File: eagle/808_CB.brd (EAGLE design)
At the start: 100 x 80 mm, 56 parts, among them IC1 4584N, IC2 TL072P, Q1 2N3904, Q2 2N3904, Q3 2N3904, Q4 2N3906, X1 22-23-2021

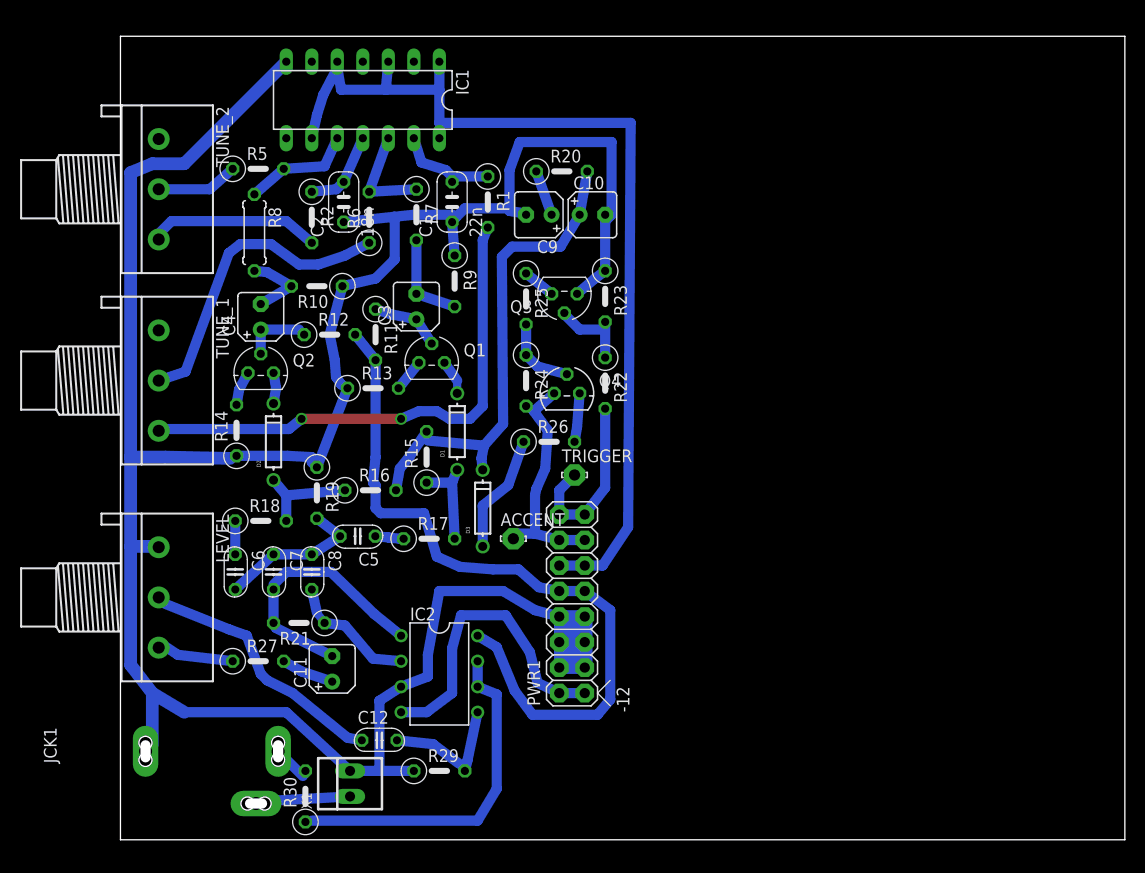
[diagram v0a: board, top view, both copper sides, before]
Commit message: tweaks and cleanups
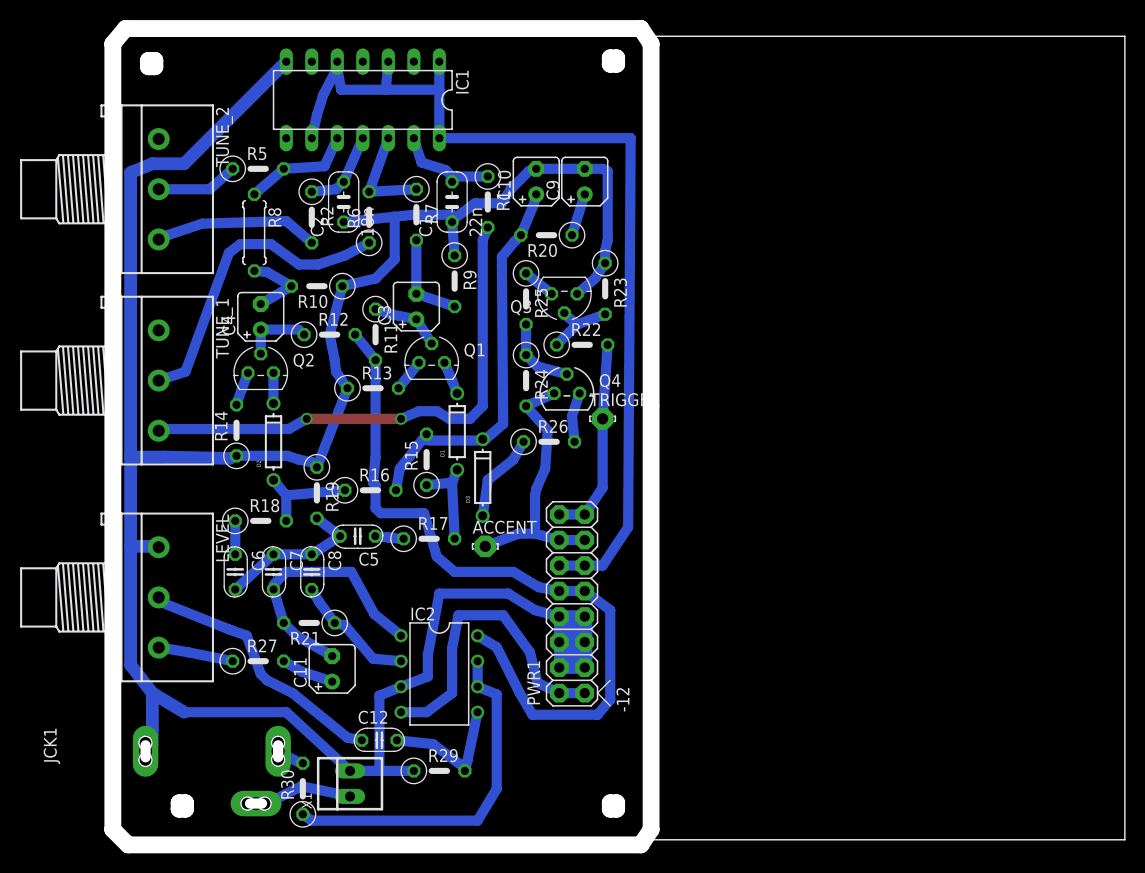
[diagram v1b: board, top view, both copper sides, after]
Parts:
- moved R20 6.53 mm to (42.4, 60.2), turned to 180 degrees
- moved C10 6.49 mm to (41.4, 65.5), turned to 90 degrees
- moved TRIGGER 6.25 mm to (48.0, 41.9)
- moved C9 5.64 mm to (46.2, 65.5), turned to 90 degrees
- moved R22 4.44 mm to (46.0, 49.3), turned to 0 degrees
- moved D3 3.05 mm to (36.1, 36.1)
- moved ACCENT 2.90 mm to (36.3, 29.2)
- moved R21 1.02 mm to (18.8, 21.6)
- moved R30 0.80 mm to (18.2, 5.08)
- moved R23 0.76 mm to (48.3, 54.9)
- moved R15 0.25 mm to (30.5, 37.8)
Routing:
- net GND: track 262.4 -> 250.9 mm
- net N$17: track 49.6 -> 39.3 mm
- net TRIG*: track 23.9 -> 27.0 mm
- net N$19: track 11.9 -> 8.89 mm
- net LT: track 18.3 -> 20.0 mm
- net +5V: track 98.7 -> 97.2 mm
- net N$517: track 8.93 -> 7.60 mm
- net CY_OUT: track 4.05 -> 2.76 mm
- net N$29: track 8.34 -> 7.54 mm
- net N$8: track 17.1 -> 16.3 mm
- net N$26: track 12.8 -> 12.2 mm
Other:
- board size 100 x 80 mm -> 100.8 x 81.3 mm
